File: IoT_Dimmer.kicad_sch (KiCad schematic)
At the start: 52 parts, among them J1 Screw_Terminal_01x02, J2 Screw_Terminal_01x02, J3 Conn_01x06_Pin, SW1 RotaryEncoder_Switch_MP, U1 MOC3021S, U2 VOS628AT, U3 ESP32-C6FH4, Y2 Crystal_GND24

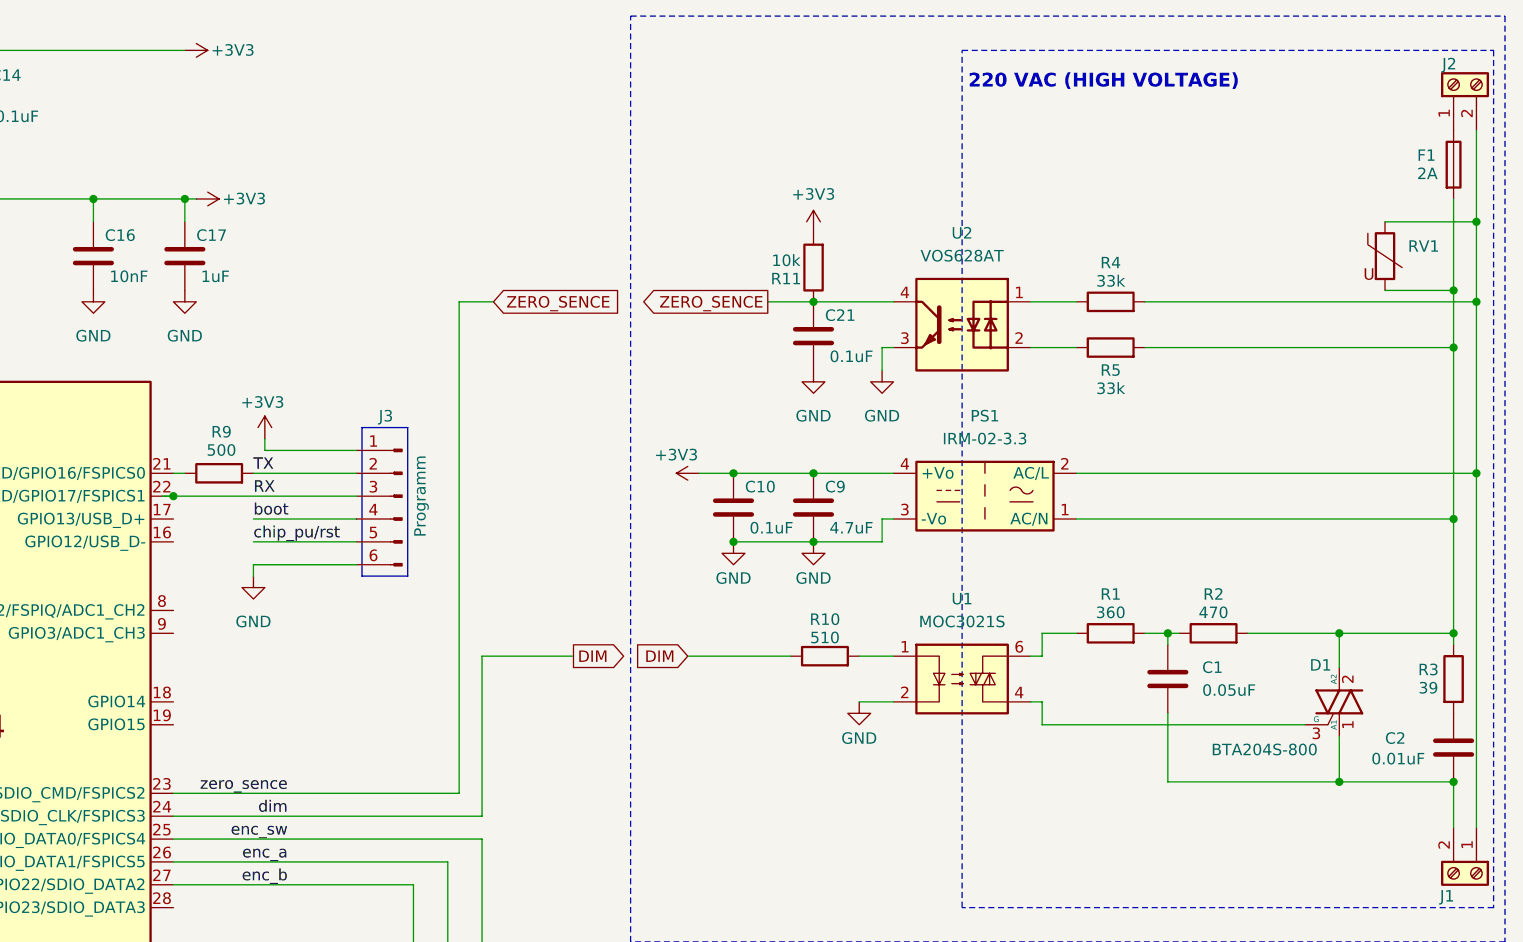
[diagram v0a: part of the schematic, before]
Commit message: PCB_start
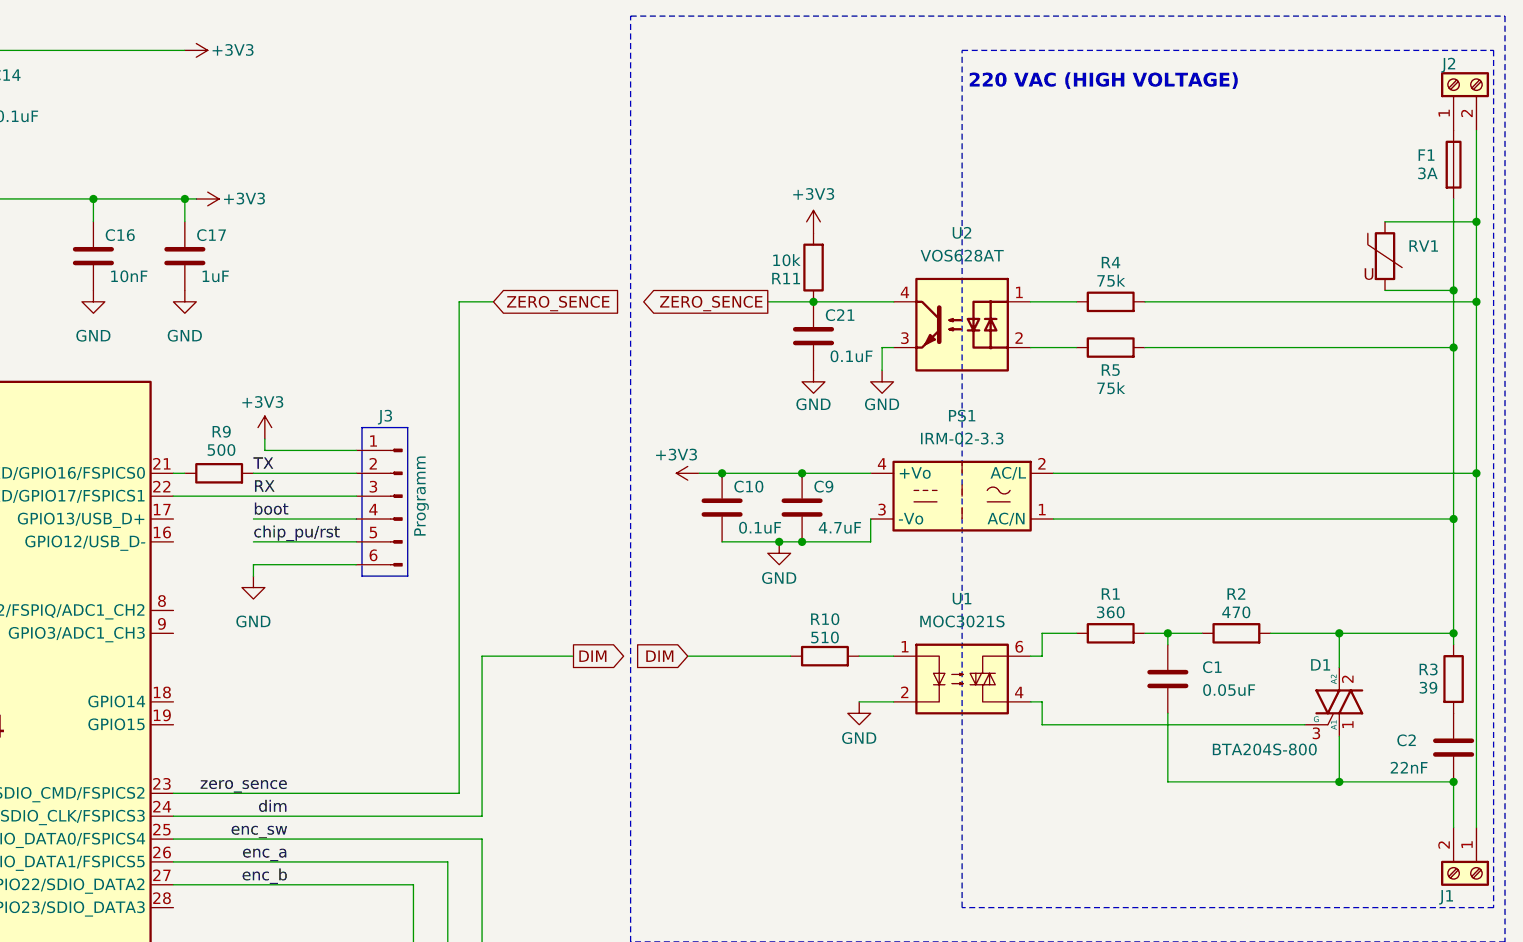
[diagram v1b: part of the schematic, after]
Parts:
- C1: footprint (none) -> Capacitor_SMD:C_1812_4532Metric
- C10, C11, C12, C13, C14, C15, C16, C17, C18, C19, C20, C21, C5, C6, C7, C8, C9: footprint Capacitor_SMD:C_0805_2012Metric -> Capacitor_SMD:C_0603_1608Metric
- C2: value 0.01uF -> 22nF; footprint (none) -> Capacitor_SMD:C_1812_4532Metric
- C3, C4: footprint (none) -> Capacitor_SMD:C_0603_1608Metric
- F1: value 2A -> 3A
- J1: value Screw_Terminal_01x02 -> Wago_2059-302998-403:CONN2_2059-302&slash_998-403_WAG
- J2: footprint (none) -> Wago_2059-302998-403:CONN2_2059-302&slash_998-403_WAG
- L1, L2: footprint (none) -> Inductor_SMD:L_0805_2012Metric
- R1, R2, R3: footprint Resistor_SMD:R_0805_2012Metric -> Resistor_SMD:R_1206_3216Metric
- R10, R11, R12, R13, R14, R6, R7, R8, R9: footprint Resistor_SMD:R_0805_2012Metric -> Resistor_SMD:R_0603_1608Metric
- R4, R5: value 33k -> 75k; footprint (none) -> Resistor_SMD:R_1206_3216Metric
- RV1: footprint Varistor:Varistor_Panasonic_VF -> Varistor:RV_Disc_D7mm_W3.4mm_P5mm
- SW1: value RotaryEncoder_Switch_MP -> EVE-SBBFE516B
- Y2: footprint (none) -> Crystal:Crystal_SMD_2016-4Pin_2.0x1.6mm
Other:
- moved on the sheet: C10, C9, PS1, R2
